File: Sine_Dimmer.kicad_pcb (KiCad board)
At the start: 2 copper layers, 31 parts, among them J1 Screw_Terminal_01x03, J2 Screw_Terminal_01x03, Q1 IPW60R037P7, Q2 IPW60R037P7, U1 UCC20520, U2 ESP-12E

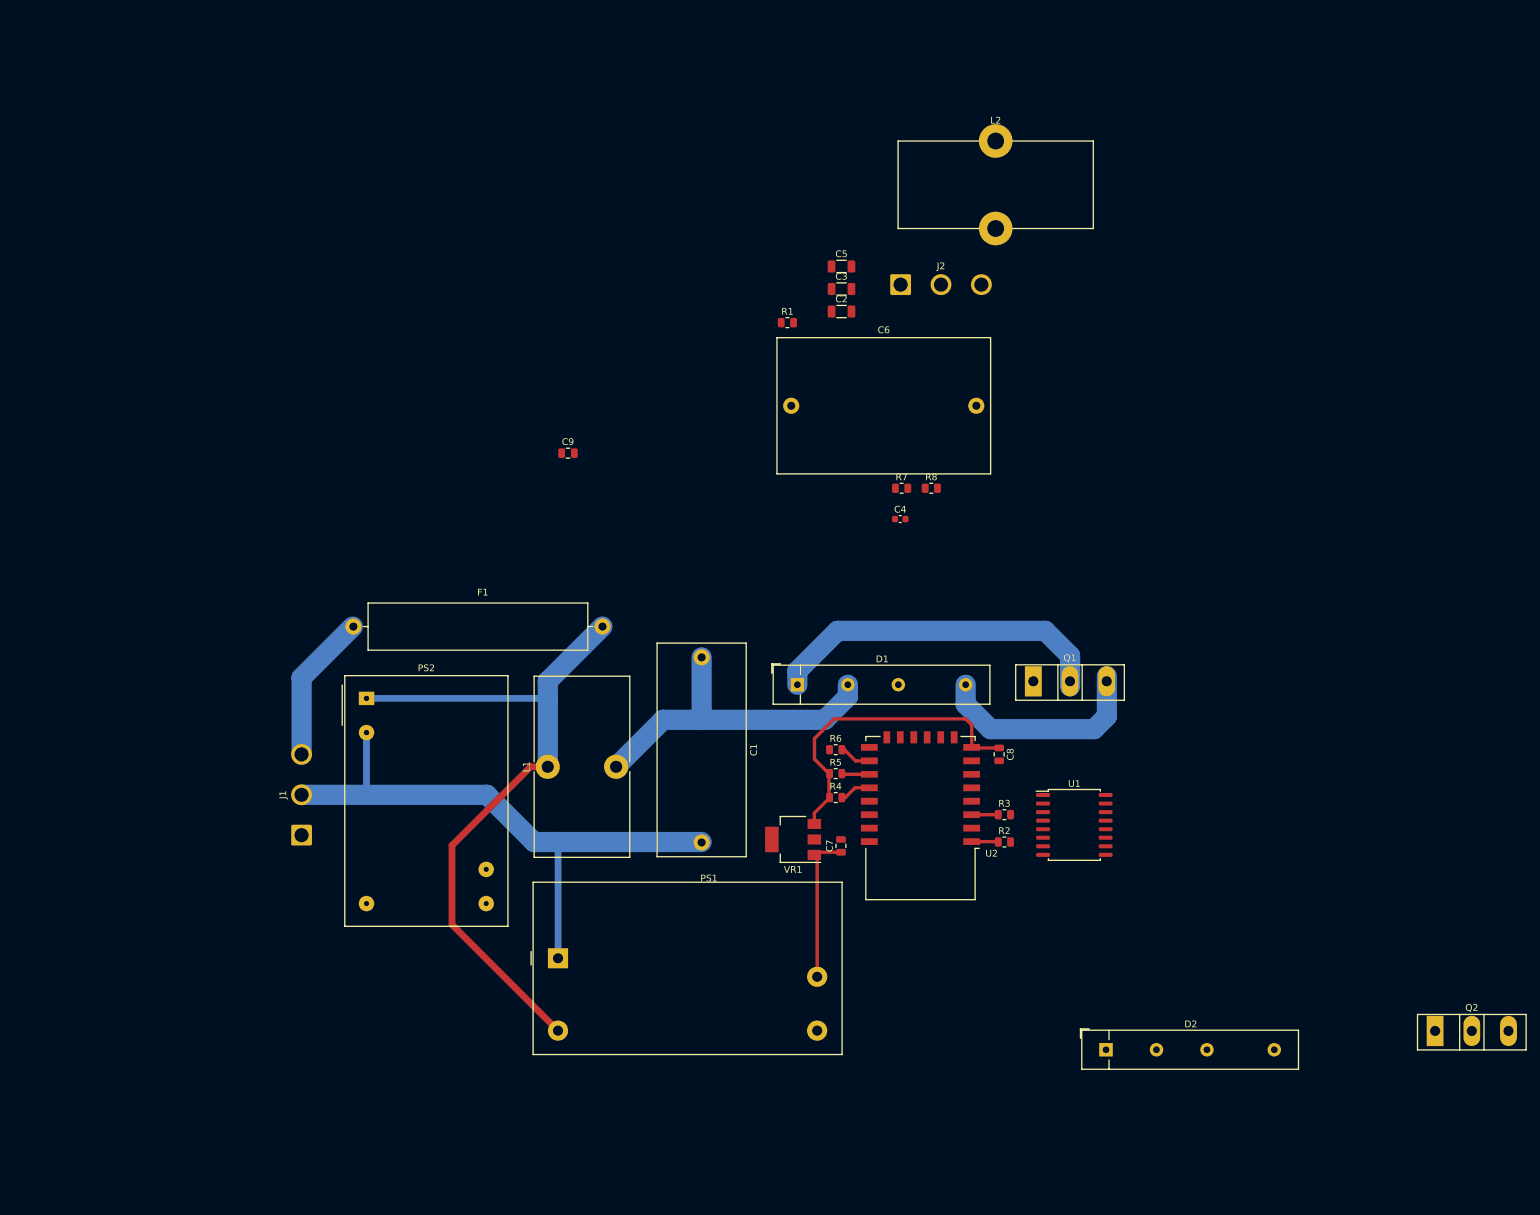
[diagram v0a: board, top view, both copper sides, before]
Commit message: 1
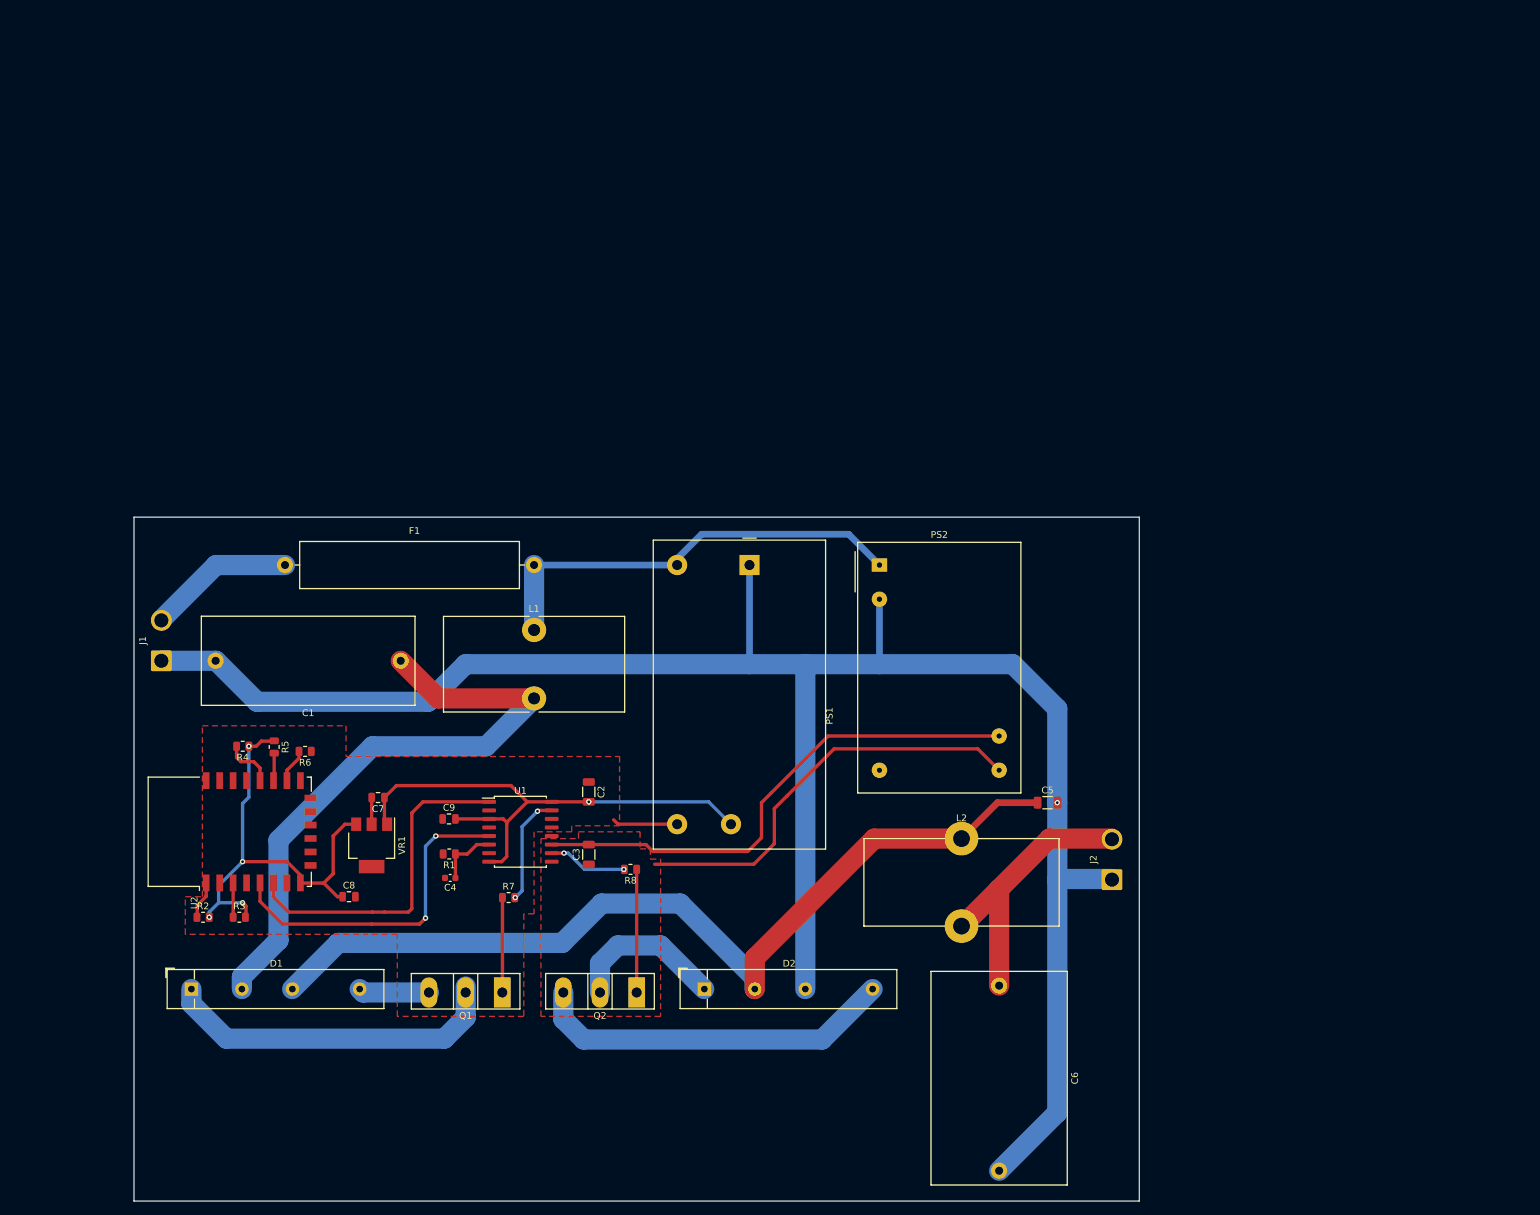
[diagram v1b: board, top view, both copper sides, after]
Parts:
- J1, J2: value Screw_Terminal_01x03 -> Screw_Terminal_01x02; footprint Connector_Wire:SolderWire-1.5sqmm_1x03_P6mm_D1.7mm_OD3mm -> Connector_Wire:SolderWire-1.5sqmm_1x02_P6mm_D1.7mm_OD3mm
- moved R2 119.6 mm to (81.4, 110.7)
- moved Q2 118.8 mm to (145.8, 121.9), turned to 180 degrees
- moved R3 114.7 mm to (86.8, 110.7)
- moved L2 103.8 mm to (194.1, 99.1)
- moved U2 102.6 mm to (85.3, 98.0), turned to 90 degrees
- moved D1 100.7 mm to (79.6, 121.4)
- moved C8 98.9 mm to (103.1, 107.7), turned to 0 degrees
- moved J2 93.8 mm to (216.4, 105.2), turned to 90 degrees
- moved R1 93.6 mm to (118.0, 101.3), turned to 180 degrees
- moved C3 92.0 mm to (138.7, 101.4), turned to 90 degrees
- moved C6 91.5 mm to (199.6, 120.9), turned to 270 degrees
- moved Q1 91.4 mm to (125.8, 121.9), turned to 180 degrees
- moved R4 88.4 mm to (87.3, 85.3), turned to 180 degrees
- moved C4 85.5 mm to (118.1, 104.9), turned to 180 degrees
- moved C5 85.3 mm to (206.8, 93.7)
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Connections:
- J1 pad 1: Net-(J1-Pad1) -> Net-(C1-Pad2)
- J1 pad 2: Net-(C1-Pad2) -> Net-(F1-Pad2)
- J2 pad 1: Net-(J1-Pad1) -> Net-(C1-Pad2)
- J2 pad 2: Net-(C1-Pad2) -> Net-(C6-Pad1)
- U1 pad 3: Net-(U1-Pad3) -> VCC
- U1 pad 8: Net-(U1-Pad8) -> VCC
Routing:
- net Net-(C1-Pad2): track 88.9 -> 293.7 mm, vias 0 -> 1
- net Net-(C5-Pad1): track 0.00 -> 136.4 mm
- net Net-(C3-Pad1): track 0.00 -> 116.9 mm
- net Net-(C3-Pad2): track 0.00 -> 77.0 mm
- net VCC: track 22.4 -> 78.9 mm, vias 0 -> 1
- net pwm: track 0.00 -> 50.1 mm
- net dis: track 0.00 -> 49.9 mm, vias 0 -> 2
- net Net-(C1-Pad1): track 49.8 -> 93.2 mm
- net Net-(C6-Pad1): track 0.00 -> 42.1 mm
- net Net-(F1-Pad1): track 104.2 -> 65.3 mm
- net Net-(D2-Pad1): track 0.00 -> 23.6 mm
- net Net-(C8-Pad1): track 46.8 -> 67.2 mm, vias 0 -> 4
- net Net-(Q2-Pad1): track 0.00 -> 18.3 mm
- net Net-(R7-Pad2): track 0.00 -> 16.4 mm, vias 0 -> 2
- net Net-(Q1-Pad1): track 0.00 -> 14.1 mm
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- added copper zone on F.Cu, net GND
- added copper zone on F.Cu, net Net-(C3-Pad1)
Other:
- board outline added: 149.4 x 101.6 mm

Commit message: 1
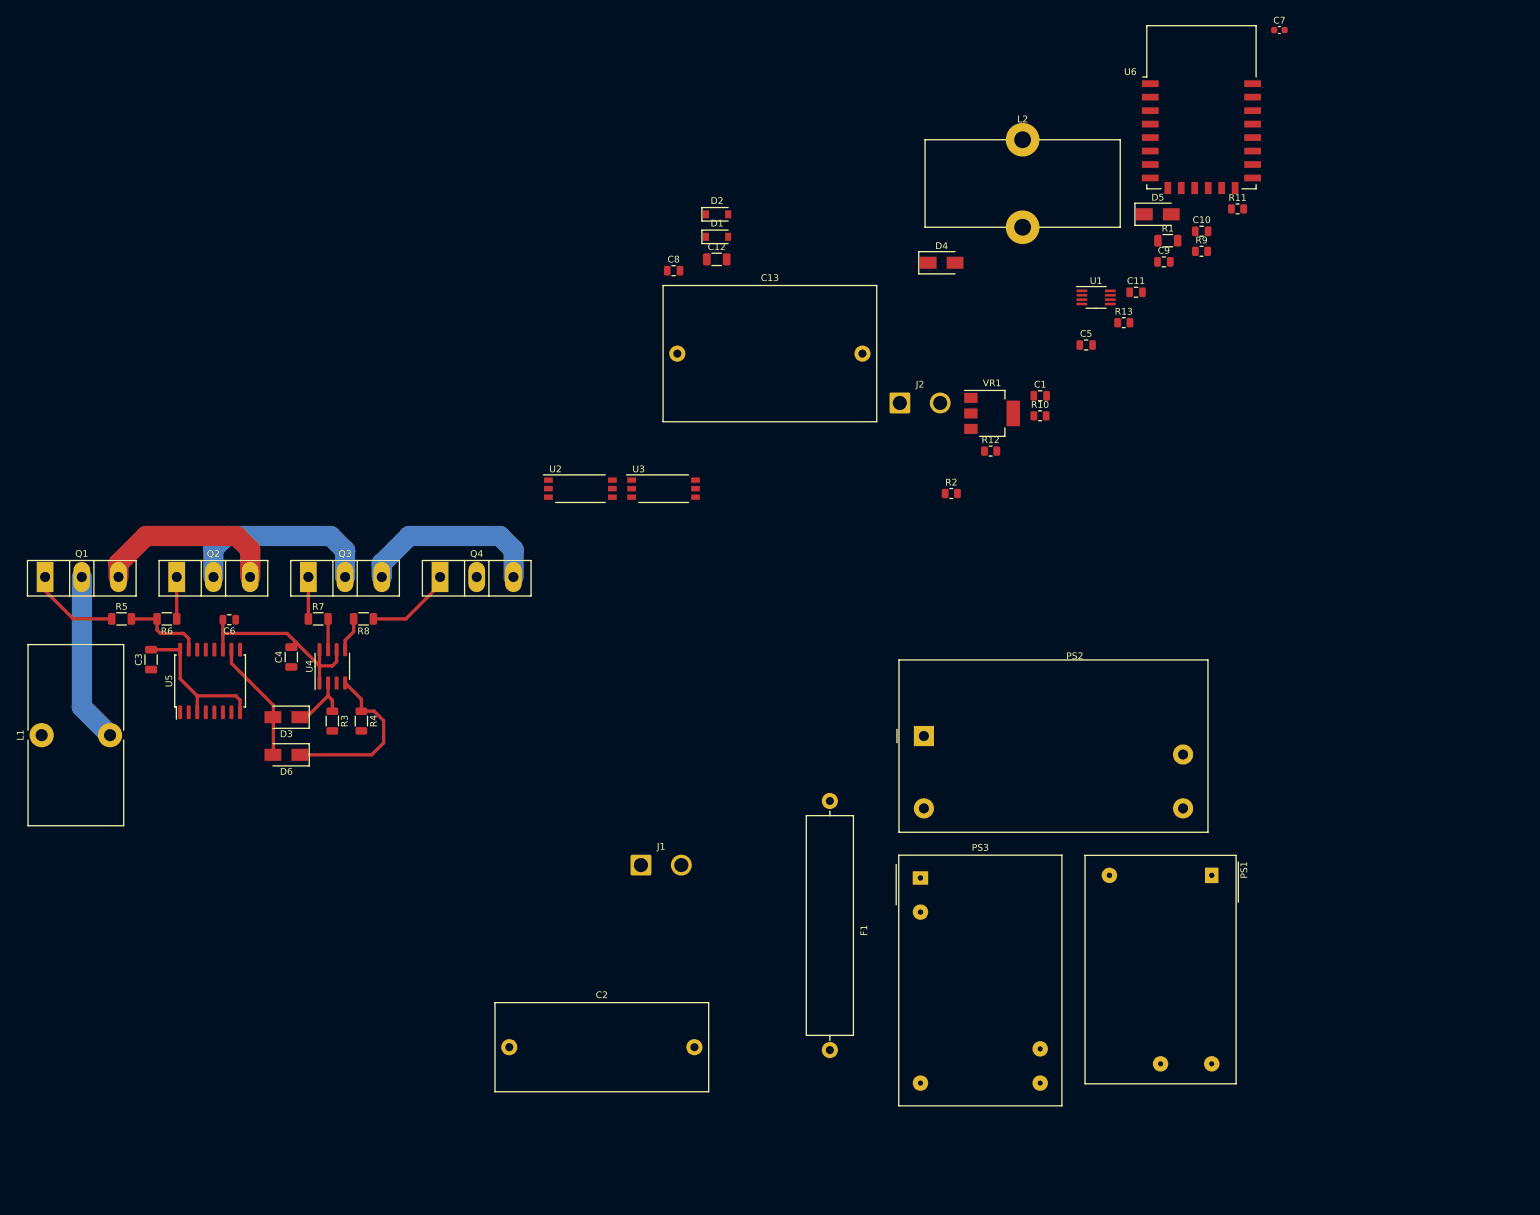
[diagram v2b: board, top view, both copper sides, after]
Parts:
- added C10: 1u, Capacitor_SMD:C_0805_2012Metric, F.Cu at (229.7, 8.83)
- added C11: 1u, Capacitor_SMD:C_0805_2012Metric, F.Cu at (220.0, 17.9)
- added C12: 2.2n, Capacitor_SMD:C_1206_3216Metric, F.Cu at (157.7, 13.0)
- added C13: 10u, Capacitor_THT:C_Rect_L31.5mm_W20.0mm_P27.50mm_MKS4, F.Cu at (151.8, 27.0)
- added D3: D, Diode_SMD:D_SMA, F.Cu at (93.8, 81.0)
- added D4: D, Diode_SMD:D_SMA, F.Cu at (191.1, 13.5)
- added D5: D, Diode_SMD:D_SMA, F.Cu at (223.2, 6.31)
- added D6: D, Diode_SMD:D_SMA, F.Cu at (93.8, 86.6)
- added PS3: IRM-03-12, Converter_ACDC:Converter_ACDC_MeanWell_IRM-03-xx_THT, F.Cu at (188.0, 104.9)
- added Q3: IPW60R037P7, Package_TO_SOT_THT:TO-247-3_Vertical, F.Cu at (97.0, 60.2)
- added Q4: IPW60R037P7, Package_TO_SOT_THT:TO-247-3_Vertical, F.Cu at (116.6, 60.2)
- added R10: 3.3k, Resistor_SMD:R_0805_2012Metric, F.Cu at (205.7, 36.3)
- added R11: 3.3k, Resistor_SMD:R_0805_2012Metric, F.Cu at (235.1, 5.51)
- added R12: 3.3k, Resistor_SMD:R_0805_2012Metric, F.Cu at (198.4, 41.5)
- added R13: 3.3k, Resistor_SMD:R_0805_2012Metric, F.Cu at (218.2, 22.4)
- added R9: 3.3k, Resistor_SMD:R_0805_2012Metric, F.Cu at (229.7, 11.8)
- added U3: TLP2745, Package_SO:SO-6L_10x3.84mm_P1.27mm, F.Cu at (149.8, 47.1)
- added U4: 2EDN7424F, Package_SO:SOIC-8_3.9x4.9mm_P1.27mm, F.Cu at (100.6, 73.5)
- added U5: UCC20520, Package_SO:SOIC-16W_7.5x10.3mm_P1.27mm, F.Cu at (82.4, 75.6)
- added U6: ESP-12E, RF_Module:ESP-12E, F.Cu at (229.7, -9.59)
- C1: value 4.7u -> 1u; footprint Capacitor_THT:C_Rect_L31.5mm_W13.0mm_P27.50mm_MKS4 -> Capacitor_SMD:C_0805_2012Metric
- C2: value 2.2u -> 4.7u; footprint Capacitor_SMD:C_1206_3216Metric -> Capacitor_THT:C_Rect_L31.5mm_W13.0mm_P27.50mm_MKS4
- C4: value 0.1u -> 2.2u; footprint Capacitor_SMD:C_0603_1608Metric -> Capacitor_SMD:C_1206_3216Metric
- C5: value 2.2n -> 1u; footprint Capacitor_SMD:C_1206_3216Metric -> Capacitor_SMD:C_0805_2012Metric
- C6: value 10u -> 1u; footprint Capacitor_THT:C_Rect_L31.5mm_W20.0mm_P27.50mm_MKS4 -> Capacitor_SMD:C_0805_2012Metric
- C7: value 1u -> 0.1u; footprint Capacitor_SMD:C_0805_2012Metric -> Capacitor_SMD:C_0603_1608Metric
- D1, D2: value D_Bridge_+AA- -> 3; footprint Diode_THT:Diode_Bridge_32.0x5.6x17.0mm_P10.0mm_P7.5mm -> Diode_SMD:D_SOD-123
- J1: value Screw_Terminal_01x02 -> Input
- J2: value Screw_Terminal_01x02 -> Output
- PS1: value IRM-05-12 -> IRM-02-5; footprint Converter_ACDC:Converter_ACDC_MeanWell_IRM-05-xx_THT -> Converter_ACDC:Converter_ACDC_MeanWell_IRM-02-xx_THT
- PS2: value IRM-03-12 -> IRM-05-12; footprint Converter_ACDC:Converter_ACDC_MeanWell_IRM-03-xx_THT -> Converter_ACDC:Converter_ACDC_MeanWell_IRM-05-xx_THT
- R1: value 5.1k -> 100k; footprint Resistor_SMD:R_0805_2012Metric -> Resistor_SMD:R_1206_3216Metric
- R2: value 3.3k -> 5.1k
- R3, R4: value 3.3k -> 1k; footprint Resistor_SMD:R_0805_2012Metric -> Resistor_SMD:R_1206_3216Metric
- R5, R6: value 3.3k -> 0; footprint Resistor_SMD:R_0805_2012Metric -> Resistor_SMD:R_1206_3216Metric
- R7, R8: footprint Resistor_SMD:R_0805_2012Metric -> Resistor_SMD:R_1206_3216Metric
- U1: value UCC20520 -> LT1711; footprint Package_SO:SOIC-16W_7.5x10.3mm_P1.27mm -> Package_SO:MSOP-8_3x3mm_P0.65mm
- U2: value ESP-12E -> TLP2745; footprint RF_Module:ESP-12E -> Package_SO:SO-6L_10x3.84mm_P1.27mm
- moved C7 175.9 mm to (241.3, -21.1), turned to 0 degrees
- moved R1 140.3 mm to (224.7, 10.2), turned to 0 degrees
- moved D1 136.3 mm to (157.7, 9.66)
- moved C9 134.6 mm to (224.1, 13.4)
- moved R2 127.7 mm to (192.5, 47.8)
- moved C6 126.6 mm to (85.3, 66.5), turned to 180 degrees
- moved U1 116.7 mm to (214.1, 18.7)
- moved D2 115.1 mm to (157.7, 6.31)
- moved VR1 112.3 mm to (198.6, 35.9), turned to 0 degrees
- moved C8 104.8 mm to (151.3, 14.7)
- moved L2 104.2 mm to (203.1, -4.76)
- moved C1 102.8 mm to (205.7, 33.3), turned to 0 degrees
- moved Q2 92.1 mm to (77.5, 60.2), turned to 0 degrees
- moved Q1 91.8 mm to (57.9, 60.2), turned to 0 degrees
- moved F1 84.4 mm to (174.5, 130.5), turned to 90 degrees
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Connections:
- C1 pad 1: Net-(C1-Pad1) -> NEUT
- C2 pad 1: GND -> Net-(C2-Pad1)
- C2 pad 2: VCC -> NEUT
- C3 pad 1: Net-(C3-Pad1) -> GND
- C3 pad 2: Net-(C3-Pad2) -> VCC
- C4 pad 1: Net-(C4-Pad1) -> VSS
- C4 pad 2: GND -> VDD
- C5 pad 1: Net-(C5-Pad1) -> GND
- C5 pad 2: Net-(C1-Pad2) -> VCC
- C6 pad 1: Net-(C6-Pad1) -> VSS
- C6 pad 2: Net-(C1-Pad2) -> VDD
- C7 pad 1: VCC -> Net-(C7-Pad1)
- C8 pad 1: Net-(C8-Pad1) -> VSS
- C8 pad 2: GND -> VDD
- C9 pad 1: GND -> VDD
- C9 pad 2: VCC -> VSS
- D1 pad 2: Net-(C1-Pad1) -> Net-(D1-Pad2)
- D2 pad 1: Net-(D2-Pad1) -> Net-(D1-Pad1)
- D2 pad 2: Net-(C5-Pad1) -> NEUT
- F1 pad 1: Net-(F1-Pad1) -> LINE
- J1 pad 1: Net-(C1-Pad2) -> NEUT
- J2 pad 1: Net-(C1-Pad2) -> NEUT
- J2 pad 2: Net-(C6-Pad1) -> VPP
- L1 pad 1: Net-(F1-Pad1) -> LINE
- L1 pad 2: Net-(C1-Pad1) -> Net-(C2-Pad1)
- L2 pad 1: Net-(C5-Pad1) -> Net-(C12-Pad1)
- L2 pad 2: Net-(C6-Pad1) -> VPP
- PS1 pad 1: Net-(C1-Pad2) -> NEUT
- PS1 pad 2: Net-(F1-Pad1) -> LINE
- PS1 pad 3: GND -> NEUT
- PS1 pad 4: VCC -> Net-(C1-Pad2)
- PS2 pad 1: Net-(F1-Pad1) -> NEUT
- PS2 pad 3: Net-(C1-Pad2) -> GND
- Q1 pad 2: Net-(D1-Pad1) -> Net-(C2-Pad1)
- Q2 pad 2: Net-(D2-Pad1) -> Net-(C12-Pad1)
- Q2 pad 3: Net-(C3-Pad1) -> GND
- R1 pad 1: Net-(C4-Pad1) -> Net-(D1-Pad2)
- R1 pad 2: GND -> LINE
- R2 pad 1: Net-(R2-Pad1) -> Net-(C7-Pad1)
- R2 pad 2: Net-(C8-Pad1) -> GND
- R3 pad 1: Net-(R3-Pad1) -> Net-(D3-Pad1)
- R3 pad 2: Net-(C8-Pad1) -> VSS
- R4 pad 1: Net-(C8-Pad1) -> Net-(D5-Pad1)
- R4 pad 2: Net-(R4-Pad2) -> VSS
- R5 pad 1: Net-(C8-Pad1) -> Net-(Q1-Pad1)
- R6 pad 1: GND -> Net-(Q2-Pad1)
- R6 pad 2: Net-(R6-Pad2) -> Net-(R5-Pad2)
- R7 pad 1: Net-(Q1-Pad1) -> Net-(Q3-Pad1)
- R8 pad 1: Net-(Q2-Pad1) -> Net-(Q4-Pad1)
- U1 pad 1: pwm -> Net-(C1-Pad2)
- U1 pad 2: (no net) -> Net-(D1-Pad2)
- U1 pad 3: VCC -> NEUT
- U1 pad 4: GND -> NEUT
- U1 pad 5: dis -> NEUT
- U1 pad 6: Net-(C4-Pad1) -> NEUT
- U1 pad 7: (no net) -> Net-(U1-Pad7)
- U1 pad 8: VCC -> Net-(U1-Pad8)
- U2 pad 1: Net-(R2-Pad1) -> Net-(U1-Pad8)
- U2 pad 3: Net-(R3-Pad1) -> NEUT
- U2 pad 4: Net-(U2-Pad4) -> VSS
- U2 pad 5: dis -> rev
- U2 pad 6: pwm -> VDD
- VR1 pad 3: Net-(C8-Pad1) -> Net-(C11-Pad1)
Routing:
- net Net-(C1-Pad2): track 293.7 -> 0.00 mm, vias 1 -> 0
- net Net-(C5-Pad1): track 136.4 -> 0.00 mm
- net Net-(C3-Pad1): track 116.9 -> 0.00 mm
- net Net-(C1-Pad1): track 93.2 -> 0.00 mm
- net Net-(C3-Pad2): track 77.0 -> 0.00 mm
- net Net-(C8-Pad1): track 67.2 -> 0.00 mm, vias 4 -> 0
- net Net-(F1-Pad1): track 65.3 -> 0.00 mm
- net VCC: track 78.9 -> 23.2 mm, vias 1 -> 0
- net Net-(D1-Pad1): track 51.0 -> 0.00 mm
- net pwm: track 50.1 -> 0.00 mm
- net dis: track 49.9 -> 0.00 mm, vias 2 -> 0
- net Net-(C6-Pad1): track 42.1 -> 0.00 mm
- net VDD: track 0.00 -> 31.3 mm
- net Net-(C12-Pad1): track 0.00 -> 29.4 mm
- net VSS: track 0.00 -> 28.2 mm
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- removed copper zone on F.Cu, net GND
- removed copper zone on F.Cu, net Net-(C3-Pad1)
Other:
- board outline removed
